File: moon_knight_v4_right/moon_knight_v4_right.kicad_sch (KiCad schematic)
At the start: 98 parts, among them J1 AudioJack4, J2 OLED_128x32, SW1 SW_PUSH, U1 Sea-Picro

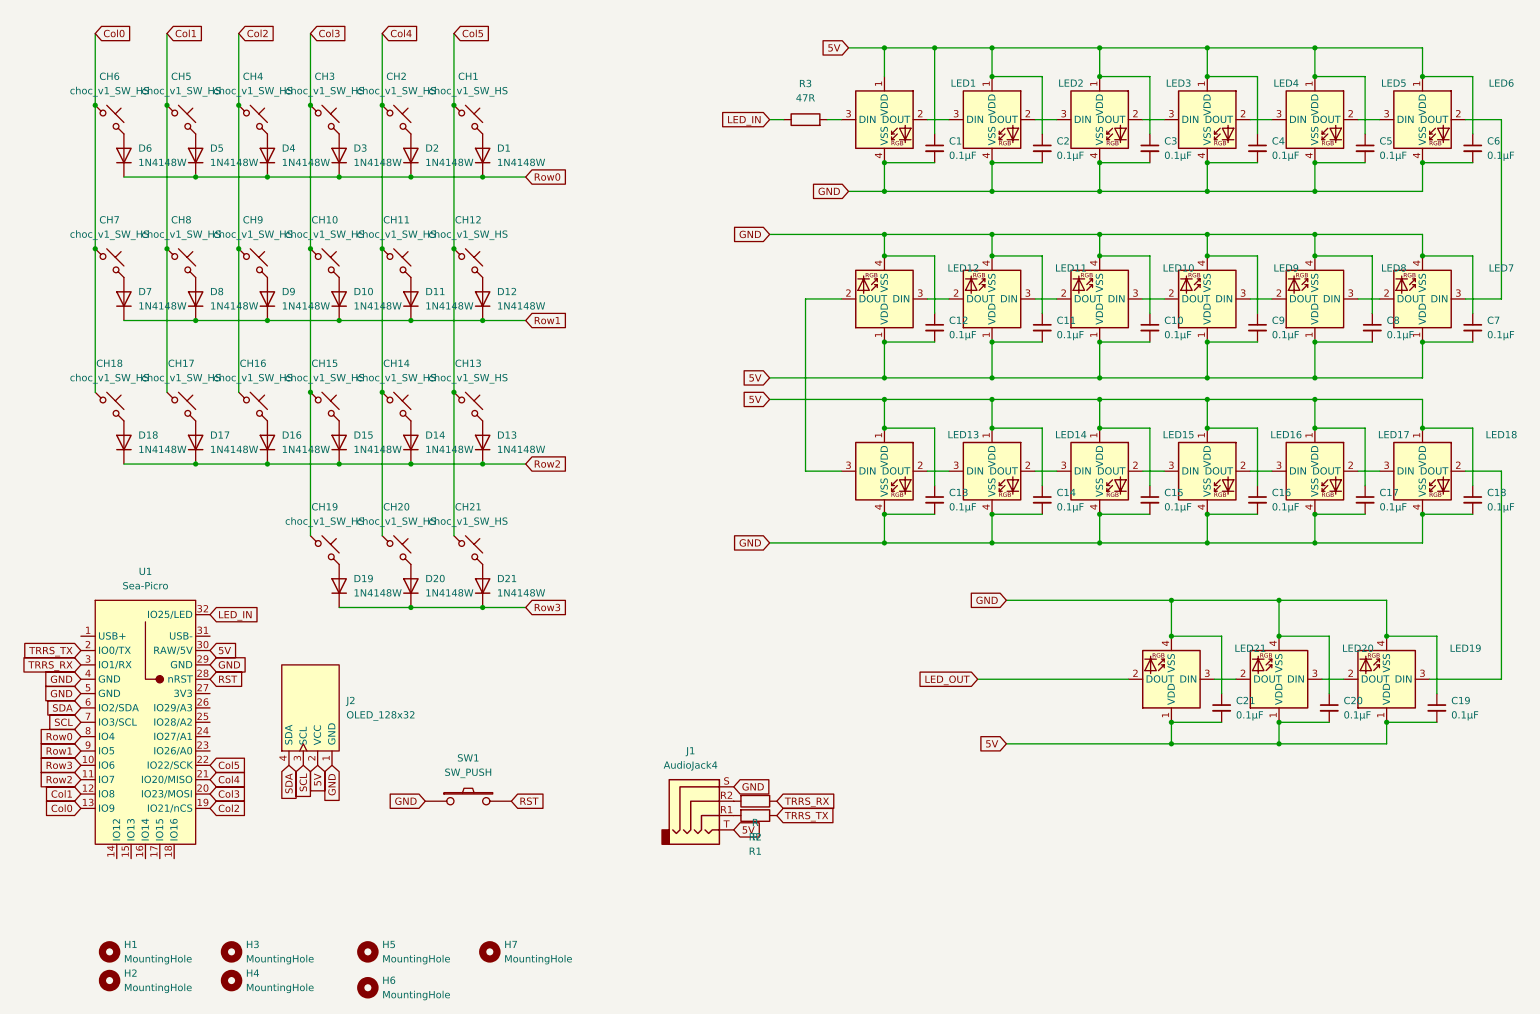
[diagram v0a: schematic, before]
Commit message: v4
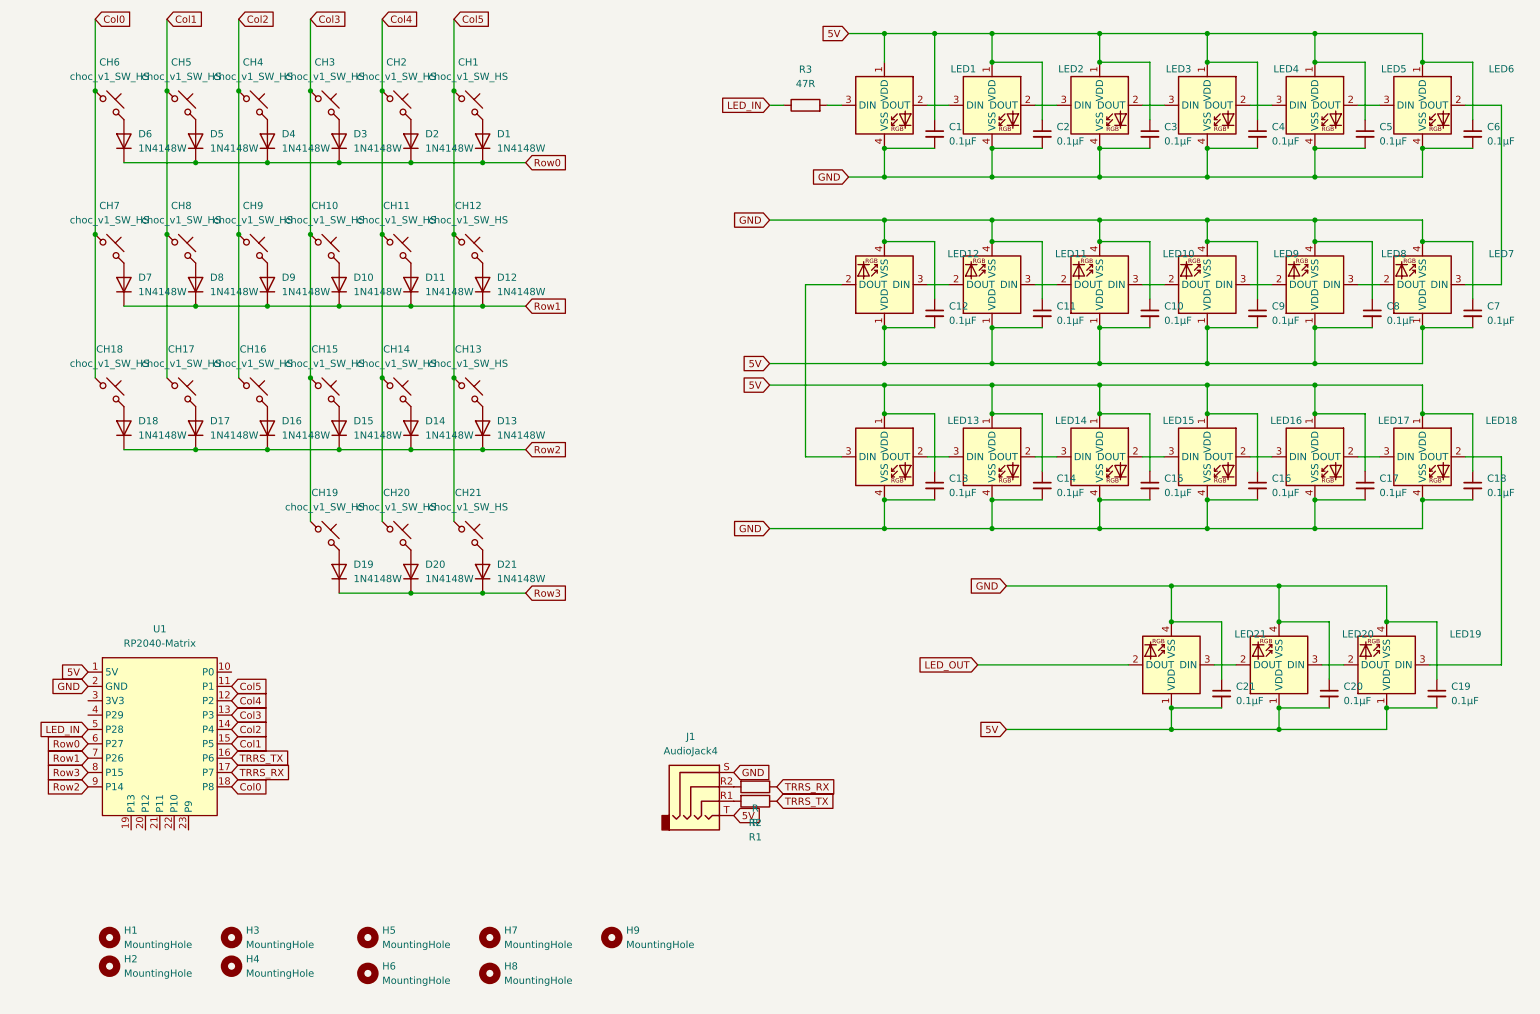
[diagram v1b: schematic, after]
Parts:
- removed J2: OLED_128x32, kleeb_display:OLED-128x32, symbol ScottoKeebs:OLED_128x32
- removed SW1: SW_PUSH, Button_Switch_SMD:SW_SPST_TS-1088-xR020, symbol kbd:SW_PUSH
- removed U1: Sea-Picro, josh-module:Sea-Picro_EXT_Module_Flipped, symbol josh-module:Sea-Picro
- added H8, H9: MountingHole, MountingHole:MountingHole_2.2mm_M2, symbol Mechanical:MountingHole
- added U1: RP2040-Matrix, PCM_marbastlib-xp-promicroish:RP2040-Matrix_AH, symbol PCM_marbastlib-promicroish:RP2040-Matrix
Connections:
- net 5V: now also U1.1 (5V)
- net Col0: now also U1.18 (P8)
- net Col1: now also U1.15 (P5)
- net Col2: now also U1.14 (P4)
- net Col3: now also U1.13 (P3)
- net Col4: now also U1.12 (P2)
- net Col5: now also U1.11 (P1)
- net GND: now also U1.2 (GND)
- net LED_IN: now also U1.5 (P28)
- net Row0: now also U1.6 (P27)
- net Row1: now also U1.7 (P26)
- net Row2: now also U1.9 (P14)
- net Row3: now also U1.8 (P15)
- net TRRS_RX: now also U1.17 (P7)
- net TRRS_TX: now also U1.16 (P6)
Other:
- moved on the sheet: C1, C10, C11, C12, C13, C14, C15, C16, C17, C18, C19, C2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
